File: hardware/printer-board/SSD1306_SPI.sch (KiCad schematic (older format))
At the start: 2 parts

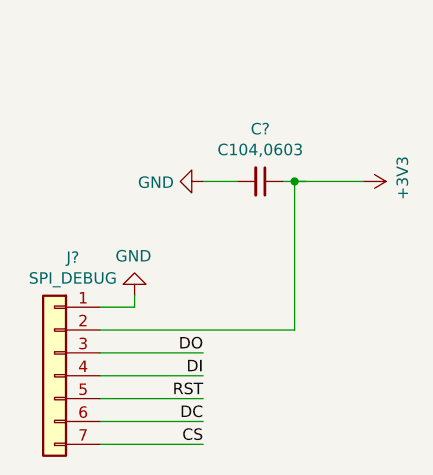
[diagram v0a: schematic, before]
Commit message: update ROUTING,
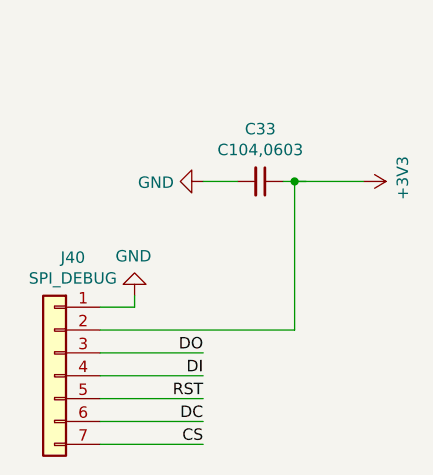
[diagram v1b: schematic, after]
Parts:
- gave numbers to parts that had none: 2
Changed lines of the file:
@@
 P 6050 4150
 AR Path="/5CC8321E/5CE3C56F" Ref="J?"  Part="1"
-AR Path="/5CE3BAD7/5CE3C56F" Ref="J?"  Part="1"
-F 0 "J?" H 5970 4667 50  0000 C CNN
+AR Path="/5CE3BAD7/5CE3C56F" Ref="J40"  Part="1"
+F 0 "J40" H 5970 4667 50  0000 C CNN
 F 1 "SPI_DEBUG" H 5970 4576 50  0000 C CNN
 F 2 "Connector_PinHeader_1.27mm:PinHeader_1x07_P1.27mm_Vertical" H 6050 4150 50  0001 C CNN
@@
 $EndComp
 $Comp
-L power:GND #PWR?
+L power:GND #PWR0149
 U 1 1 5CE3C576
 P 6400 3800
-F 0 "#PWR?" H 6400 3550 50  0001 C CNN
+F 0 "#PWR0149" H 6400 3550 50  0001 C CNN
 F 1 "GND" H 6405 3627 50  0000 C CNN
 F 2 "" H 6400 3800 50  0001 C CNN
@@
 P 7400 3300
 AR Path="/5CC8321E/5CE3C584" Ref="#PWR?"  Part="1"
-AR Path="/5CE3BAD7/5CE3C584" Ref="#PWR?"  Part="1"
-F 0 "#PWR?" H 7400 3150 50  0001 C CNN
+AR Path="/5CE3BAD7/5CE3C584" Ref="#PWR0160"  Part="1"
+F 0 "#PWR0160" H 7400 3150 50  0001 C CNN
 F 1 "+3V3" H 7415 3473 50  0000 C CNN
 F 2 "" H 7400 3300 50  0001 C CNN
@@
 	6700 3300 6850 3300
 $Comp
-L power:GND #PWR?
+L power:GND #PWR0161
 U 1 1 5CE3C591
 P 6700 3300
-F 0 "#PWR?" H 6700 3050 50  0001 C CNN
+F 0 "#PWR0161" H 6700 3050 50  0001 C CNN
 F 1 "GND" V 6705 3172 50  0000 R CNN
 F 2 "" H 6700 3300 50  0001 C CNN
@@
 $EndComp
 $Comp
-L taobao-c:C104,0603 C?
+L taobao-c:C104,0603 C33
 U 1 1 5CE3C58A
 P 6950 3300
-F 0 "C?" V 6721 3300 50  0000 C CNN
+F 0 "C33" V 6721 3300 50  0000 C CNN
 F 1 "C104,0603" V 6812 3300 50  0000 C CNN
 F 2 "Capacitor_SMD:C_0603_1608Metric_Pad1.05x0.95mm_HandSolder" H 6950 3300 50  0001 C CNN

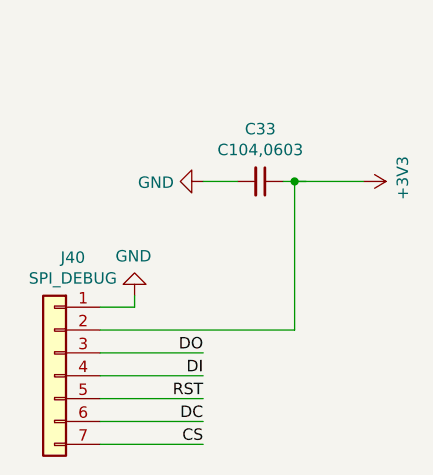
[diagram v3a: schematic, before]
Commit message: update ROUTING,
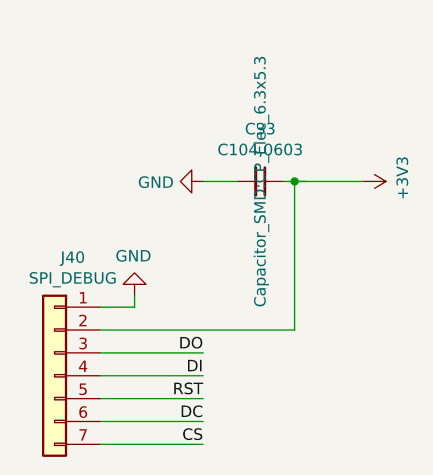
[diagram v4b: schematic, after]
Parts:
- C33: footprint Capacitor_SMD:C_0603_1608Metric_Pad1.05x0.95mm_HandSolder -> Capacitor_SMD:CP_Elec_6.3x5.3
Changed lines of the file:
@@
 F 0 "C33" V 6721 3300 50  0000 C CNN
 F 1 "C104,0603" V 6812 3300 50  0000 C CNN
-F 2 "Capacitor_SMD:C_0603_1608Metric_Pad1.05x0.95mm_HandSolder" H 6950 3300 50  0001 C CNN
+F 2 "Capacitor_SMD:CP_Elec_6.3x5.3" H 6950 3300 50  0000 C CNN
 F 3 "~" H 6950 3300 50  0001 C CNN
 	1    6950 3300
